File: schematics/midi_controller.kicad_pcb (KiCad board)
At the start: 2 copper layers, 60 x 45 mm, 9 parts, among them U1 4051

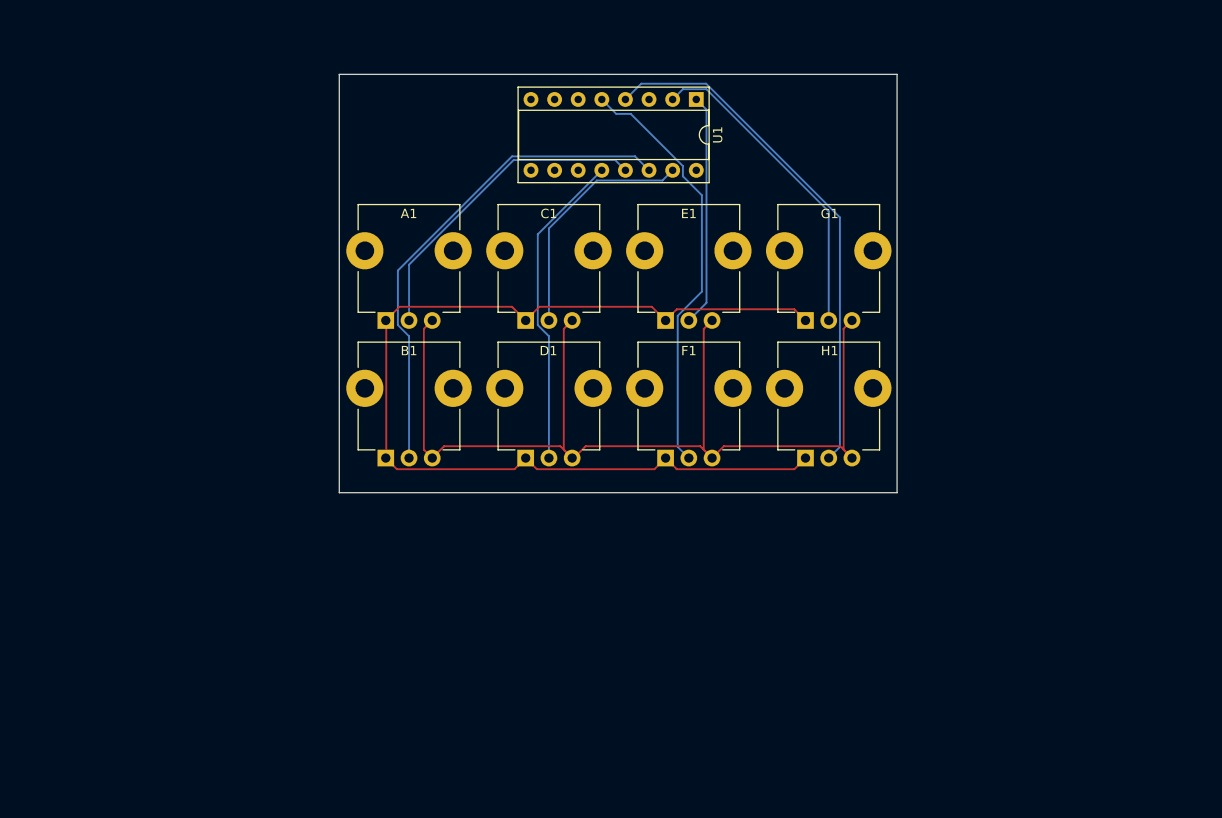
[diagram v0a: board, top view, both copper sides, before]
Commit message: fixing stuff
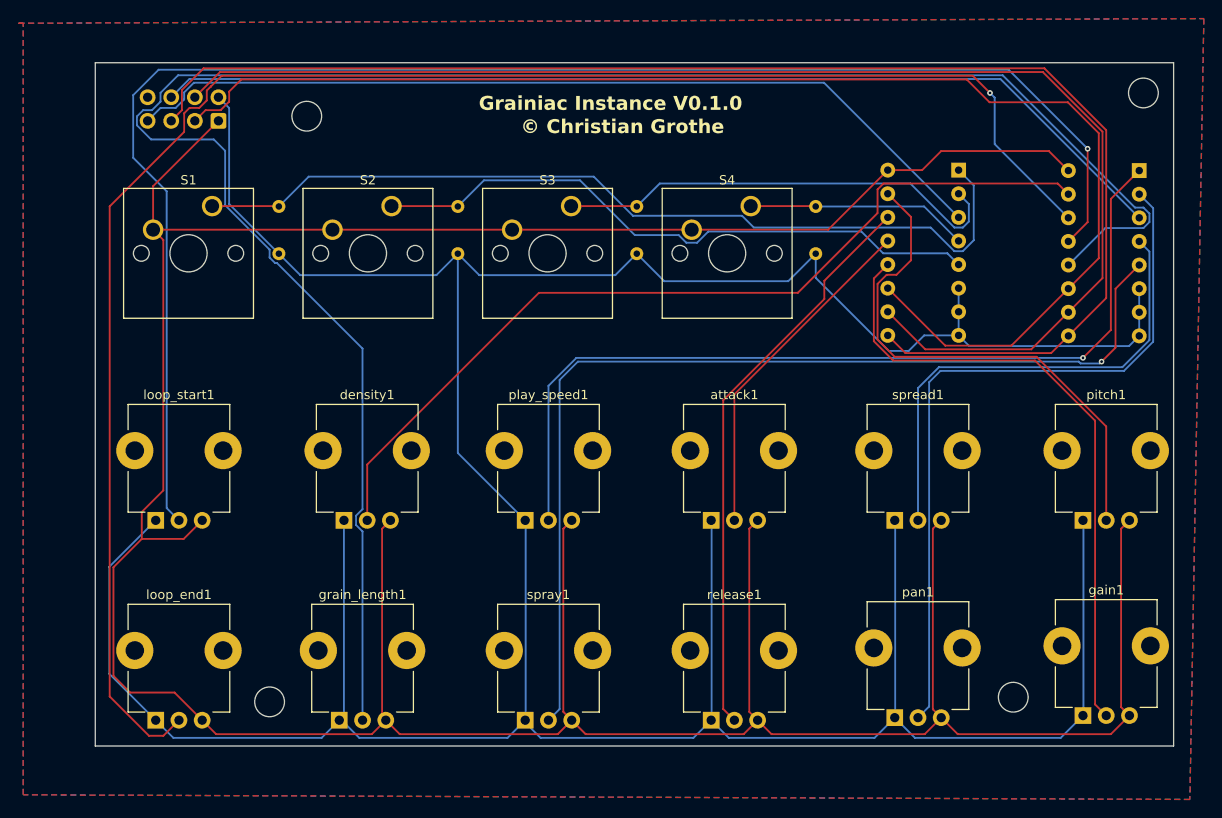
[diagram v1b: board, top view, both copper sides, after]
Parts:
- removed A1, B1, C1, D1, E1, F1, G1, H1: Pot, Potentiometer_THT:Potentiometer_TT_P0915N
- added J1: Conn_01x08_Pin, Connector_IDC:IDC-Header_2x04_P2.54mm_Vertical, B.Cu at (112.0, 55.0)
- added R1: 1.5K, Resistor_THT:R_Axial_DIN0204_L3.6mm_D1.6mm_P5.08mm_Horizontal, B.Cu at (118.5, 64.2)
- added R2: 1.5K, Resistor_THT:R_Axial_DIN0204_L3.6mm_D1.6mm_P5.08mm_Horizontal, B.Cu at (137.8, 64.2)
- added R3: 1.5K, Resistor_THT:R_Axial_DIN0204_L3.6mm_D1.6mm_P5.08mm_Horizontal, B.Cu at (157.0, 64.2)
- added R4: 1.5K, Resistor_THT:R_Axial_DIN0204_L3.6mm_D1.6mm_P5.08mm_Horizontal, B.Cu at (176.2, 64.2)
- added S1: Record, Button_Switch_Keyboard:SW_Cherry_MX_1.00u_PCB, F.Cu at (111.3, 64.2)
- added S2: Hold, Button_Switch_Keyboard:SW_Cherry_MX_1.00u_PCB, F.Cu at (130.6, 64.2)
- added S3: Play Dir, Button_Switch_Keyboard:SW_Cherry_MX_1.00u_PCB, F.Cu at (149.9, 64.2)
- added S4: Grain Dir, Button_Switch_Keyboard:SW_Cherry_MX_1.00u_PCB, F.Cu at (169.3, 64.2)
- added U3: 4051, Package_DIP:DIP-16_W7.62mm_Socket, B.Cu at (191.6, 60.3)
- added attack1: ~, Potentiometer_THT:Potentiometer_TT_P0915N, F.Cu at (165.0, 98.0)
- added density1: ~, Potentiometer_THT:Potentiometer_TT_P0915N, F.Cu at (125.5, 98.0)
- added gain1: ~, Potentiometer_THT:Potentiometer_TT_P0915N, F.Cu at (205.0, 119.0)
- added grain_length1: ~, Potentiometer_THT:Potentiometer_TT_P0915N, F.Cu at (125.0, 119.5)
- added loop_end1: ~, Potentiometer_THT:Potentiometer_TT_P0915N, F.Cu at (105.2, 119.5)
- added loop_start1: ~, Potentiometer_THT:Potentiometer_TT_P0915N, F.Cu at (105.2, 98.0)
- added pan1: ~, Potentiometer_THT:Potentiometer_TT_P0915N, F.Cu at (184.8, 119.2)
- added pitch1: ~, Potentiometer_THT:Potentiometer_TT_P0915N, F.Cu at (205.0, 98.0)
- added play_speed1: ~, Potentiometer_THT:Potentiometer_TT_P0915N, F.Cu at (145.0, 98.0)
- added release1: ~, Potentiometer_THT:Potentiometer_TT_P0915N, F.Cu at (165.0, 119.5)
- added spray1: ~, Potentiometer_THT:Potentiometer_TT_P0915N, F.Cu at (145.0, 119.5)
- added spread1: ~, Potentiometer_THT:Potentiometer_TT_P0915N, F.Cu at (184.8, 98.0)
- U1: moved to B.Cu
- moved U1 48.3 mm to (211.1, 60.4), turned to 180 degrees
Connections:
- U1 pad 1: Pot E -> play_speed
- U1 pad 10: unconnected-(U1-B-Pad10) -> S1
- U1 pad 11: unconnected-(U1-A-Pad11) -> S0
- U1 pad 12: Pot D -> grain_length
- U1 pad 13: Pot A -> loop_start
- U1 pad 14: Pot B -> loop_end
- U1 pad 15: Pot C -> density
- U1 pad 16: unconnected-(U1-VDD-Pad16) -> +3.3V
- U1 pad 2: Pot G -> pan
- U1 pad 3: unconnected-(U1-X-Pad3) -> mux_1
- U1 pad 4: Pot H -> spread
- U1 pad 5: Pot F -> spray
- U1 pad 6: unconnected-(U1-Inh-Pad6) -> GND
- U1 pad 7: unconnected-(U1-VEE-Pad7) -> GND
- U1 pad 8: unconnected-(U1-VSS-Pad8) -> GND
- U1 pad 9: unconnected-(U1-C-Pad9) -> S2
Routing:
- net +3.3V: track 0.00 -> 403.6 mm
- net GND: track 110.5 -> 408.6 mm
- net grain_length: track 0.00 -> 208.7 mm
- net loop_end: track 0.00 -> 182.6 mm, vias 0 -> 1
- net loop_start: track 0.00 -> 165.9 mm, vias 0 -> 1
- net S2: track 0.00 -> 151.7 mm
- net S1: track 0.00 -> 145.1 mm
- net S0: track 0.00 -> 144.7 mm
- net +5V: track 111.6 -> 0.00 mm
- net mux_1: track 0.00 -> 111.1 mm
- net spray: track 0.00 -> 108.5 mm, vias 0 -> 1
- net density: track 0.00 -> 95.9 mm
- net play_speed: track 0.00 -> 95.9 mm, vias 0 -> 1
- net mux_2: track 0.00 -> 95.4 mm
- net record: track 0.00 -> 95.3 mm
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- added copper zone on B.Cu, net (none)
- added copper zone on F.Cu, net (none)
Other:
- board size 60 x 45 mm -> 116 x 73.5 mm
- board text added: "Grainiac Instance V0.1.0"
- board text added: "© Christian Grothe"
